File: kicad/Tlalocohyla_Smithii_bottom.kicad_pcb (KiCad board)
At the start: 2 copper layers, 215.7 x 90 mm, 38 parts

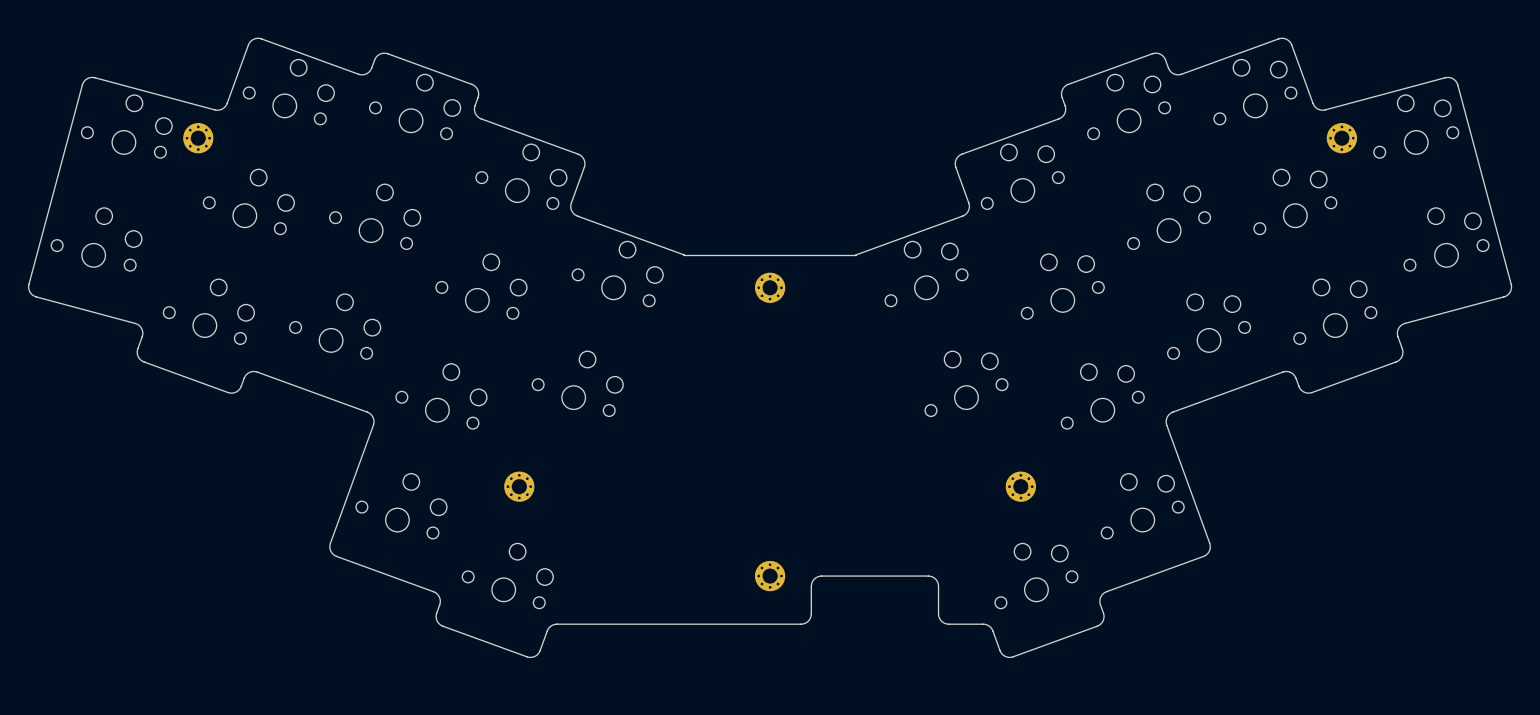
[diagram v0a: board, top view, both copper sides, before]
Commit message: Add filled zone
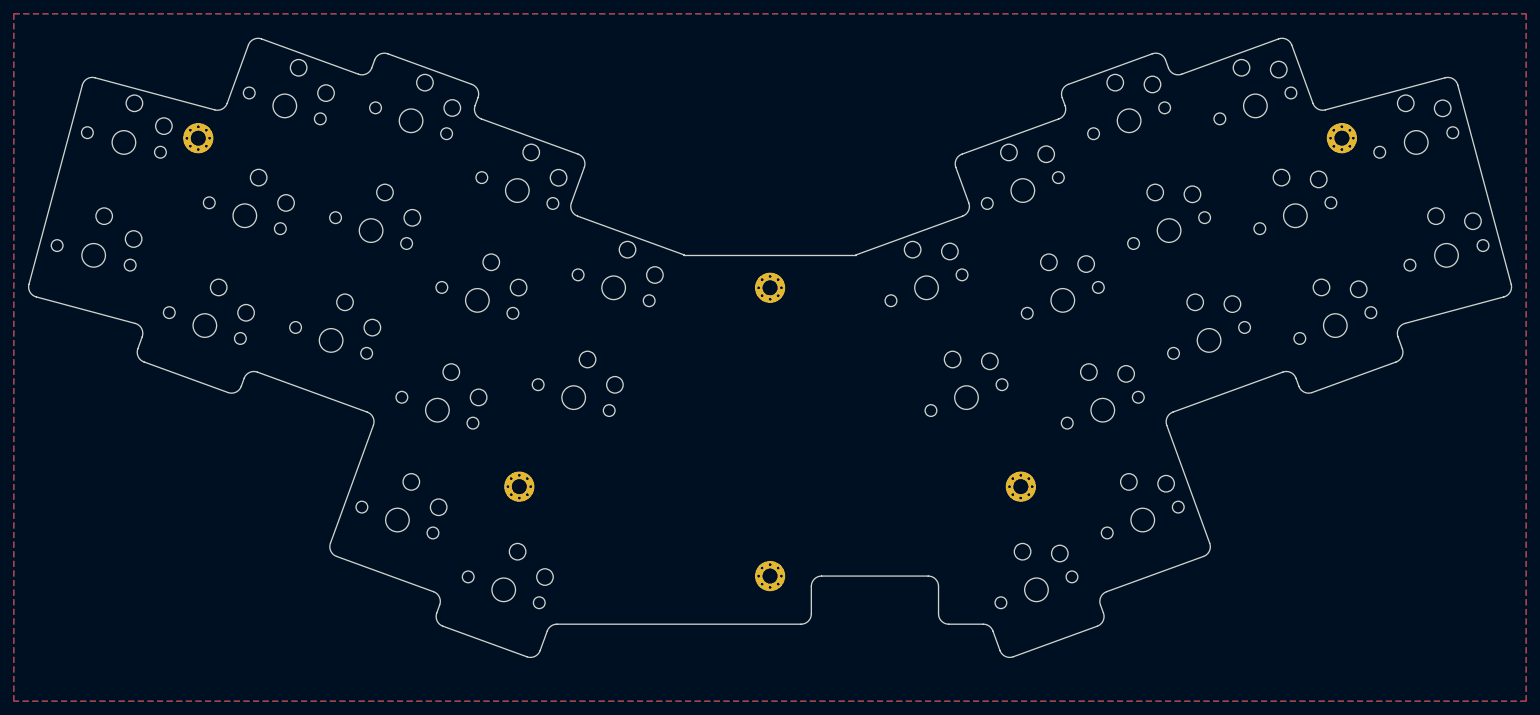
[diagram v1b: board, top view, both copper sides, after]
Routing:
- added copper zone on B.Cu, net (none)
- added copper zone on F.Cu, net (none)
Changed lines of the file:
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@@
   (gr_line (start 162.513285 75.07942) (end 162.543464 75.162337) (layer "Edge.Cuts") (width 0.15))
   (gr_arc (start 49.979881 50.373042) (mid 50.67877 49.462232) (end 51.816999 49.312382) (layer "Edge.Cuts") (width 0.15))
+  (zone (net 0) (net_name "") (layers F&B.Cu) (hatch edge 0.508)
+    (connect_pads (clearance 0.508))
+    (min_thickness 0.254) (filled_areas_thickness no)
+    (fill yes (thermal_gap 0.508) (thermal_bridge_width 0.508))
+    (polygon
+      (pts
+        (xy 260 140)
+        (xy 40 140)
+        (xy 40 40)
+        (xy 260 40)
+      )
+    )
+  )
 )
